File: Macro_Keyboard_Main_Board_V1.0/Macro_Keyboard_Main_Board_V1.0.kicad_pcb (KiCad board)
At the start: 2 copper layers, 127 x 121 mm, 87 parts, among them J1 USB_C_Receptacle_USB2.0, J2 JST SM02B-SRSS-TB(LF)(SN), J3 Conn_01x05, Q1 DMG2301L-7, SW1 SW_SPDT PCM12SMTR, SW10 SW_Push, SW11 SW_Push, SW12 SW_Push, SW13 SW_Push, SW14 SW_Push, SW15 SW_Push, SW16 SW_Push, SW17 SW_Push, SW18 SW_Push, SW19 SW_Push, SW2 SW_Push, SW20 SW_Push, SW21 SW_Push, SW22 SW_Push, SW23 SW_Push, SW3 SW_Push, SW4 SW_Push, SW5 SW_Push, SW6 SW_Push, SW7 SW_Push, SW8 SW_Push, SW9 SW_Push, U1 MCP73831T-2ACI/OT, U2 MDBT50Q-1MV2, Y1 32768Hz

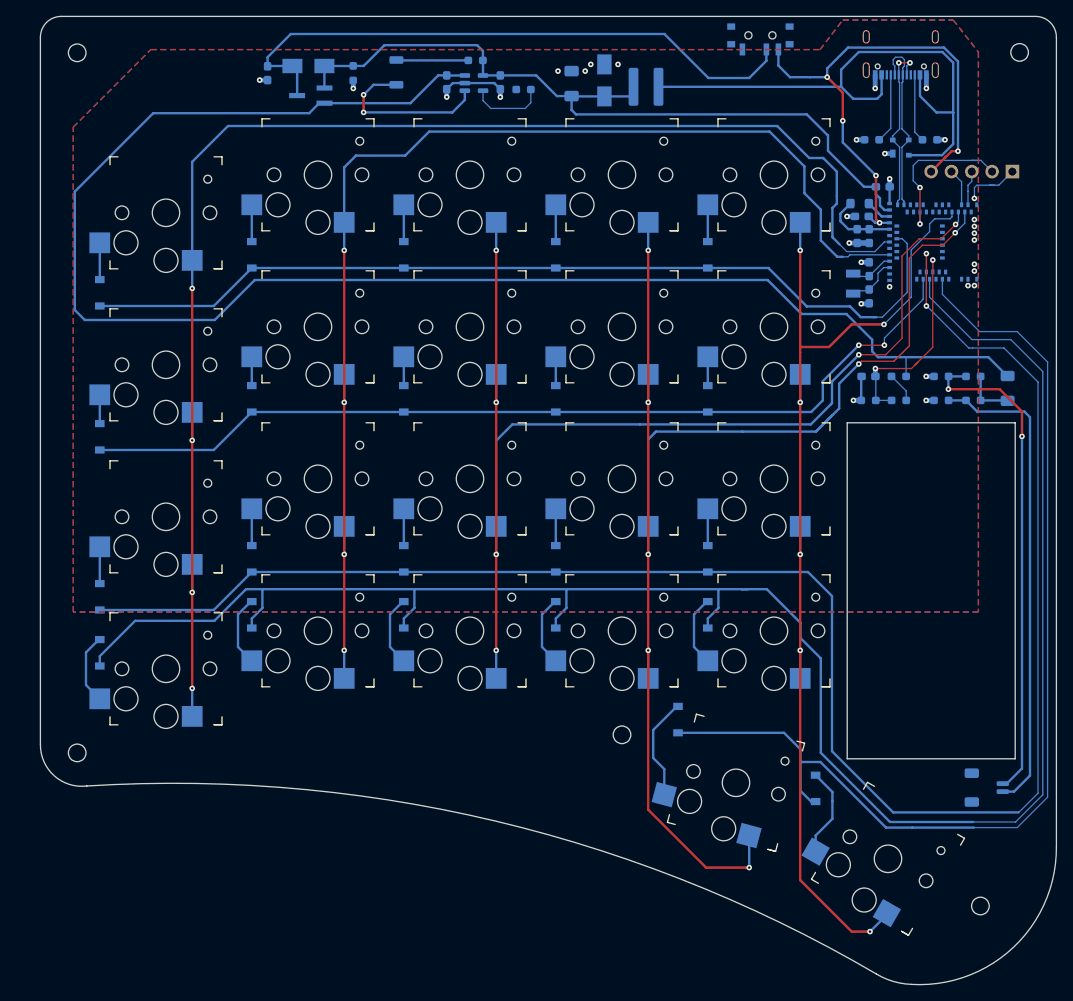
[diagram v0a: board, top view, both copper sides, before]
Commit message: Weekend changes
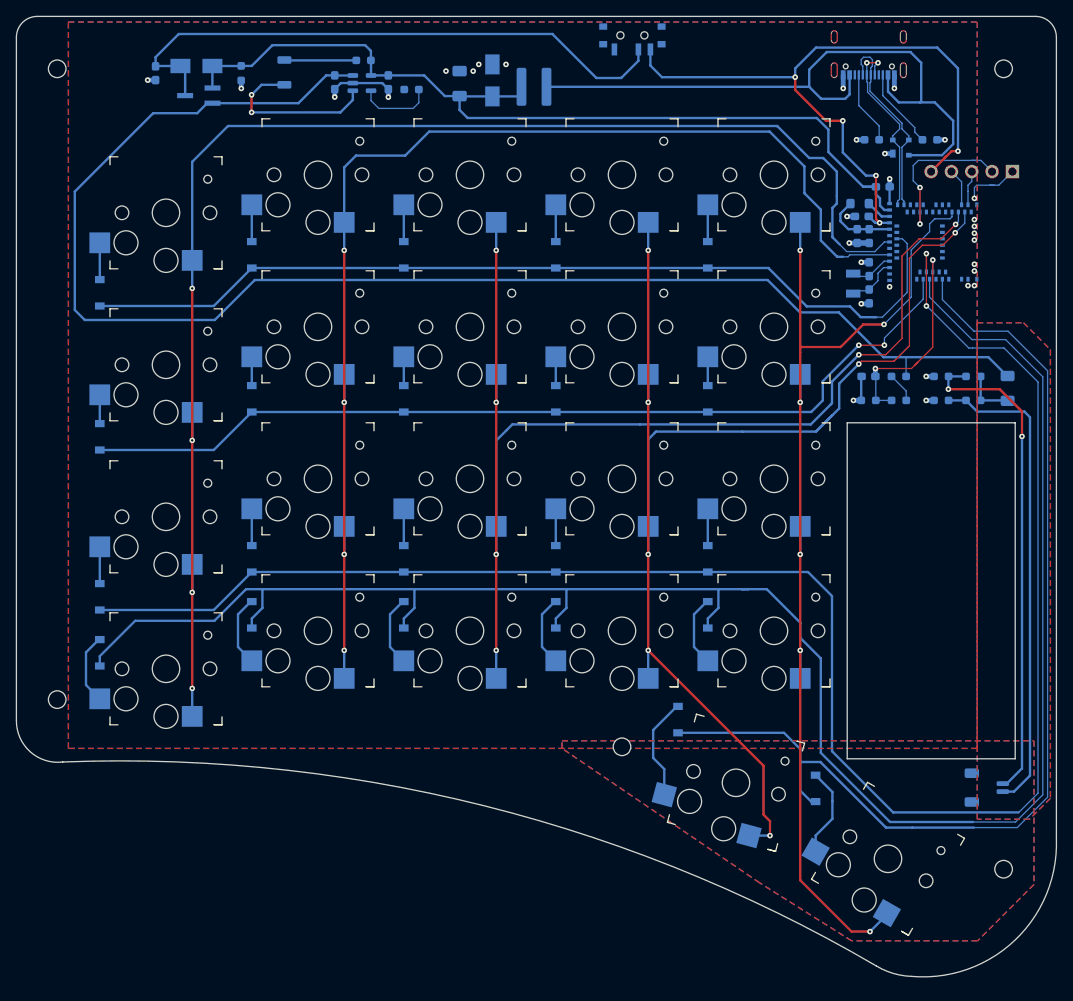
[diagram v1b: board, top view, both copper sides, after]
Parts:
- moved SW1 16.0 mm to (241.1, 105.7)
- moved C1 14.0 mm to (219.5, 111.4)
- moved C2 14.0 mm to (210.6, 111.2)
- moved C3 14.0 mm to (203.9, 111.2)
- moved C4 14.0 mm to (181.5, 110.1)
- moved D1 14.0 mm to (223.6, 111.0)
- moved D2 14.0 mm to (197.6, 110.0)
- moved D4 14.0 mm to (186.6, 109.2)
- moved Q1 14.0 mm to (186.9, 112.9)
- moved R10 14.0 mm to (192.2, 110.1)
- moved R4 14.0 mm to (213.5, 112.1)
- moved R7 14.0 mm to (207.5, 108.5)
- moved TH1 14.0 mm to (228.8, 111.8)
- moved U1 14.0 mm to (207.3, 111.3)
- moved H1 7.11 mm to (169.2, 188.4)
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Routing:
- net VDD: track 67.7 -> 86.8 mm
- net +BATT: track 197.0 -> 182.2 mm
- net VBUS: track 98.2 -> 111.8 mm
- net Net-(D3-Pad4): track 73.5 -> 85.4 mm
- net /keyboard/COL4: track 177.7 -> 170.3 mm
- net Net-(C4-Pad1): track 76.3 -> 74.3 mm
- net /keyboard/USB_N: track 22.7 -> 24.4 mm
- net /keyboard/USB_P: track 21.7 -> 23.3 mm
- net /keyboard/CC2: track 8.51 -> 10.2 mm
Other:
- board size 127 x 121 mm -> 130 x 120.1 mm
